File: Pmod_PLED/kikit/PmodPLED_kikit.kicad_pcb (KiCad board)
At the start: 2 copper layers, 88.5 x 101.3 mm, 212 parts, among them IC1 TBD62064APG, IC2 LM2940T-5.0, J1 Barrel_Jack_Switch, J3 Conn_01x03_Pin

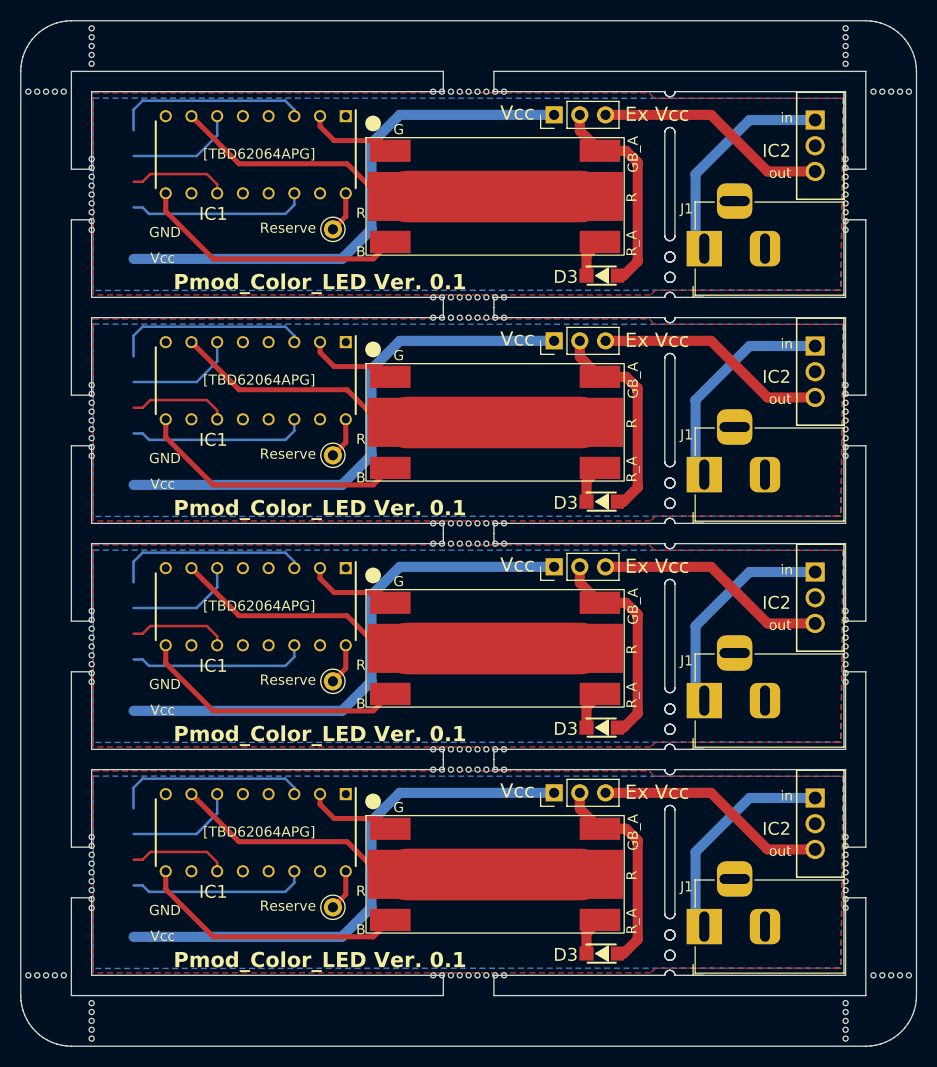
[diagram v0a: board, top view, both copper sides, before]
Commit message: 601
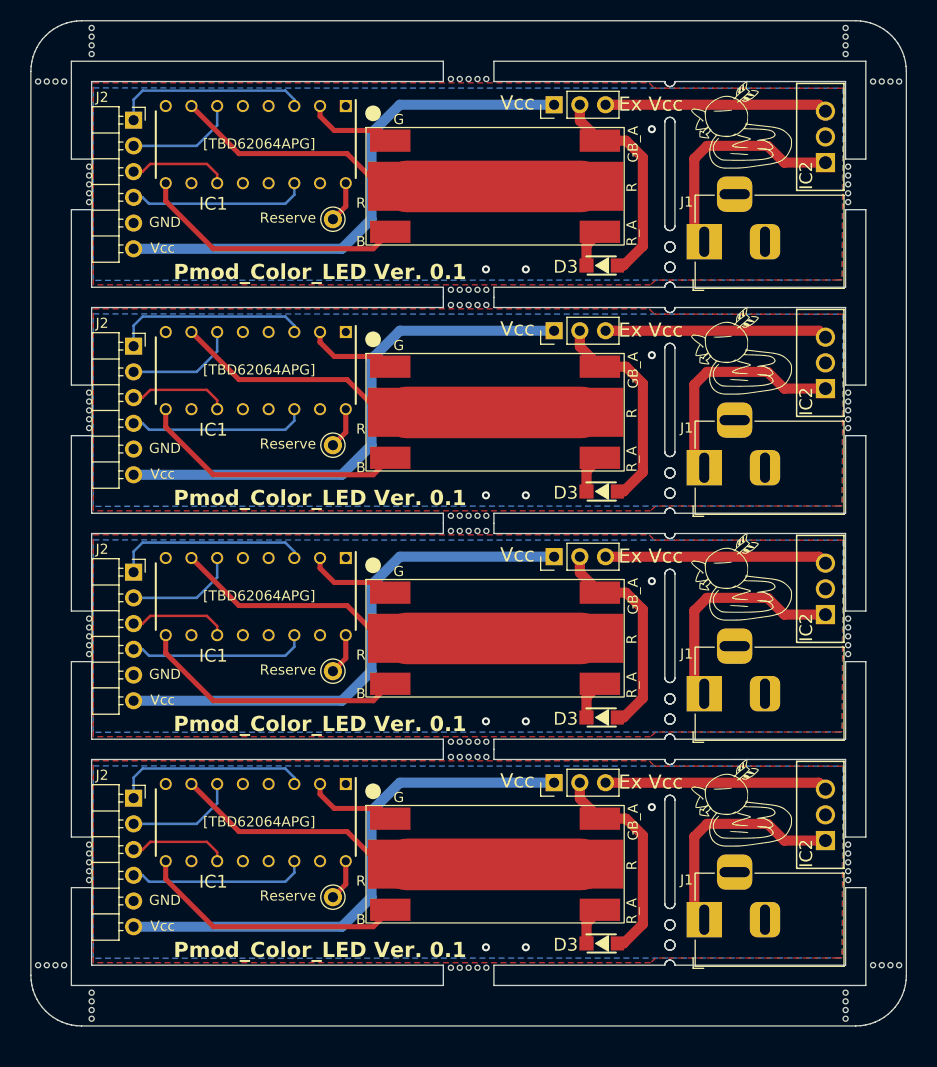
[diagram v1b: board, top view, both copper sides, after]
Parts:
- removed the D1 at (151.2, 104.3)
- removed the D1 at (151.2, 37.3)
- removed the D1 at (151.2, 59.7)
- removed the D1 at (151.2, 82.0)
- removed the D3 at (161.6, 45.2)
- removed the D3 at (161.6, 112.1)
- removed the D3 at (161.6, 89.8)
- removed the D3 at (161.6, 67.5)
- removed the IC1 at (127.5, 33.2)
- removed the IC1 at (127.5, 77.9)
- removed the IC1 at (127.5, 100.2)
- removed the IC1 at (127.5, 55.5)
- removed the IC2 at (183.7, 57.2)
- removed the IC2 at (183.7, 34.9)
- removed the IC2 at (183.7, 79.5)
- removed the IC2 at (183.7, 101.8)
- removed the J1 at (171.8, 42.5)
- removed the J1 at (171.8, 87.1)
- removed the J1 at (171.8, 109.5)
- removed the J1 at (171.8, 64.8)
- removed the J3 at (156.9, 96.2)
- removed the J3 at (156.9, 29.3)
- removed the J3 at (156.9, 73.9)
- removed the J3 at (156.9, 51.6)
- removed the REF** at (147.6, 47.3)
- removed the REF** at (111.3, 105.9)
- removed the REF** at (148.5, 47.3)
- removed the REF** at (111.3, 36.3)
- removed the REF** at (185.7, 58.6)
- removed the REF** at (147.6, 71.6)
- removed the REF** at (111.3, 63.0)
- removed the REF** at (150.2, 94.0)
- removed the REF** at (149.4, 92.0)
- removed the REF** at (185.7, 104.1)
- removed the REF** at (147.6, 49.3)
- removed the REF** at (145.0, 49.3)
- removed the REF** at (151.1, 71.6)
- removed the REF** at (145.0, 114.3)
- removed the REF** at (152.0, 71.6)
- removed the REF** at (111.3, 23.4)
- removed the REF** at (148.5, 94.0)
- removed the REF** at (192.0, 114.3)
- removed the REF** at (147.6, 94.0)
- removed the REF** at (185.7, 80.9)
- removed the REF** at (111.3, 33.7)
- removed the REF** at (148.5, 49.3)
- removed the REF** at (185.7, 85.3)
- removed the REF** at (145.9, 47.3)
- removed the REF** at (185.7, 84.4)
- removed the REF** at (111.3, 80.9)
- removed the REF** at (107.6, 114.3)
- removed the REF** at (190.2, 27.0)
- removed the REF** at (185.7, 81.8)
- removed the REF** at (111.3, 82.7)
- removed the REF** at (150.2, 27.0)
- removed the REF** at (152.0, 114.3)
- removed the REF** at (185.7, 118.8)
- removed the REF** at (145.0, 27.0)
- removed the REF** at (111.3, 118.8)
- removed the REF** at (150.2, 114.3)
- removed the REF** at (185.7, 119.6)
- removed the REF** at (145.0, 69.6)
- removed the REF** at (111.3, 79.2)
- removed the REF** at (146.8, 47.3)
- removed the REF** at (185.7, 20.8)
- removed the REF** at (185.7, 117.9)
- removed the REF** at (185.7, 38.9)
- removed the REF** at (189.4, 114.3)
- removed the REF** at (185.7, 103.2)
- removed the REF** at (185.7, 100.6)
- removed the REF** at (111.3, 57.7)
- removed the REF** at (185.7, 61.2)
- removed the REF** at (111.3, 62.1)
- removed the REF** at (152.0, 69.6)
- removed the REF** at (145.9, 94.0)
- removed the REF** at (146.8, 94.0)
- removed the REF** at (150.2, 71.6)
- removed the REF** at (152.0, 94.0)
- removed the REF** at (111.3, 21.6)
- removed the REF** at (145.9, 49.3)
- removed the REF** at (111.3, 102.4)
- removed the REF** at (111.3, 81.8)
- removed the REF** at (152.0, 27.0)
- removed the REF** at (111.3, 84.4)
- removed the REF** at (111.3, 101.5)
- removed the REF** at (147.6, 114.3)
- removed the REF** at (145.0, 94.0)
- removed the REF** at (111.3, 38.0)
- removed the REF** at (111.3, 24.2)
- removed the REF** at (191.1, 114.3)
- removed the REF** at (147.6, 92.0)
- removed the REF** at (188.5, 27.0)
- removed the REF** at (146.8, 49.3)
- removed the REF** at (111.3, 56.0)
- removed the REF** at (145.0, 47.3)
- removed the REF** at (111.3, 38.9)
- removed the REF** at (150.2, 69.6)
- removed the REF** at (185.7, 38.0)
- removed the REF** at (146.8, 92.0)
- removed the REF** at (185.7, 57.7)
- removed the REF** at (148.5, 92.0)
- removed the REF** at (185.7, 23.4)
- removed the REF** at (185.7, 107.6)
- removed the REF** at (149.4, 49.3)
- removed the REF** at (185.7, 35.4)
- removed the REF** at (185.7, 83.5)
- removed the REF** at (152.0, 92.0)
- removed the REF** at (111.3, 34.5)
- removed the REF** at (111.3, 39.8)
- removed the REF** at (185.7, 33.7)
- removed the REF** at (148.5, 69.6)
- removed the REF** at (151.1, 94.0)
- removed the REF** at (149.4, 69.6)
- removed the REF** at (147.6, 69.6)
- removed the REF** at (149.4, 71.6)
- removed the REF** at (185.7, 101.5)
- removed the REF** at (185.7, 21.6)
- removed the REF** at (146.8, 71.6)
- removed the REF** at (106.8, 27.0)
- removed the REF** at (151.1, 49.3)
- removed the REF** at (151.1, 47.3)
- removed the REF** at (185.7, 80.0)
- removed the REF** at (111.3, 107.6)
- removed the REF** at (146.8, 27.0)
- removed the REF** at (185.7, 39.8)
- removed the REF** at (149.4, 27.0)
- removed the REF** at (150.2, 92.0)
- removed the REF** at (111.3, 78.3)
- removed the REF** at (111.3, 60.4)
- removed the REF** at (111.3, 117.9)
- removed the REF** at (105.0, 27.0)
- removed the REF** at (111.3, 20.8)
- removed the REF** at (145.9, 114.3)
- removed the REF** at (185.7, 105.0)
- removed the REF** at (185.7, 40.7)
- removed the REF** at (145.9, 71.6)
- removed the REF** at (145.9, 69.6)
- removed the REF** at (148.5, 27.0)
- removed the REF** at (185.7, 106.7)
- removed the REF** at (145.0, 92.0)
- removed the REF** at (111.3, 106.7)
- removed the REF** at (190.2, 114.3)
- removed the REF** at (192.0, 27.0)
- removed the REF** at (189.4, 27.0)
- removed the REF** at (188.5, 114.3)
- removed the REF** at (185.7, 117.0)
- removed the REF** at (191.1, 27.0)
- removed the REF** at (185.7, 60.4)
- removed the REF** at (185.7, 22.5)
- removed the REF** at (149.4, 47.3)
- removed the REF** at (111.3, 37.2)
- removed the REF** at (185.7, 79.2)
- removed the REF** at (148.5, 114.3)
- removed the REF** at (185.7, 56.9)
- removed the REF** at (150.2, 49.3)
- removed the REF** at (185.7, 102.4)
- removed the REF** at (185.7, 62.1)
- removed the REF** at (185.7, 34.5)
- removed the REF** at (105.9, 27.0)
- removed the REF** at (150.2, 47.3)
- removed the REF** at (111.3, 104.1)
- removed the REF** at (149.4, 94.0)
- removed the REF** at (105.0, 114.3)
- removed the REF** at (147.6, 27.0)
- removed the REF** at (185.7, 24.2)
- removed the REF** at (185.7, 56.0)
- removed the REF** at (111.3, 35.4)
- removed the REF** at (108.5, 114.3)
- removed the REF** at (106.8, 114.3)
- removed the REF** at (105.9, 114.3)
- removed the REF** at (152.0, 49.3)
- removed the REF** at (111.3, 85.3)
- removed the REF** at (185.7, 36.3)
- removed the REF** at (185.7, 63.0)
- removed the REF** at (111.3, 59.5)
- removed the REF** at (107.6, 27.0)
- removed the REF** at (111.3, 40.7)
- removed the REF** at (185.7, 82.7)
- removed the REF** at (185.7, 105.9)
- removed the REF** at (146.8, 69.6)
- removed the REF** at (152.0, 47.3)
- removed the REF** at (111.3, 83.5)
- removed the REF** at (111.3, 100.6)
- removed the REF** at (111.3, 103.2)
- removed the REF** at (148.5, 71.6)
- removed the REF** at (111.3, 56.9)
- removed the REF** at (151.1, 114.3)
- removed the REF** at (185.7, 120.5)
- removed the REF** at (108.5, 27.0)
- removed the REF** at (111.3, 119.6)
- removed the REF** at (185.7, 78.3)
- removed the REF** at (145.0, 71.6)
- removed the REF** at (145.9, 27.0)
- removed the REF** at (146.8, 114.3)
- removed the REF** at (185.7, 37.2)
- removed the REF** at (145.9, 92.0)
- removed the REF** at (111.3, 22.5)
- removed the REF** at (111.3, 117.0)
- removed the REF** at (111.3, 120.5)
- removed the REF** at (111.3, 105.0)
- removed the REF** at (151.1, 27.0)
- removed the REF** at (111.3, 58.6)
- removed the REF** at (149.4, 114.3)
- removed the REF** at (185.7, 59.5)
- removed the REF** at (151.1, 92.0)
- removed the REF** at (111.3, 80.0)
- removed the REF** at (111.3, 61.2)
- removed the REF** at (151.1, 69.6)
- removed the Reserve at (135.1, 107.6)
- removed the Reserve at (135.1, 62.9)
- removed the Reserve at (135.1, 85.2)
- removed the Reserve at (135.1, 40.6)
- added D1: [EP204K-150G1R1B1-CA], MyLibrary:EP204-150G1R1B1-CA, F.Cu at (151.2, 58.7)
- added D1: [EP204K-150G1R1B1-CA], MyLibrary:EP204-150G1R1B1-CA, F.Cu at (151.2, 103.3)
- added D1: [EP204K-150G1R1B1-CA], MyLibrary:EP204-150G1R1B1-CA, F.Cu at (151.2, 81.0)
- added D1: [EP204K-150G1R1B1-CA], MyLibrary:EP204-150G1R1B1-CA, F.Cu at (151.2, 36.3)
- added D3: SS2040FL, SamacSys_Parts:SODFL3618X108N, F.Cu at (161.6, 66.5)
- added D3: SS2040FL, SamacSys_Parts:SODFL3618X108N, F.Cu at (161.6, 111.1)
- added D3: SS2040FL, SamacSys_Parts:SODFL3618X108N, F.Cu at (161.6, 88.8)
- added D3: SS2040FL, SamacSys_Parts:SODFL3618X108N, F.Cu at (161.6, 44.2)
- added G***: LOGO, MyLibrary:logo_kamo_ss, F.Cu at (175.4, 97.3)
- added G***: LOGO, MyLibrary:logo_kamo_ss, F.Cu at (175.4, 30.3)
- added G***: LOGO, MyLibrary:logo_kamo_ss, F.Cu at (175.4, 75.0)
- added G***: LOGO, MyLibrary:logo_kamo_ss, F.Cu at (175.4, 52.6)
- added IC1: TBD62064APG, SamacSys_Parts:DIP762W60P254L1975H445Q16N, F.Cu at (127.5, 76.9)
- added IC1: TBD62064APG, SamacSys_Parts:DIP762W60P254L1975H445Q16N, F.Cu at (127.5, 99.2)
- added IC1: TBD62064APG, SamacSys_Parts:DIP762W60P254L1975H445Q16N, F.Cu at (127.5, 54.5)
- added IC1: TBD62064APG, SamacSys_Parts:DIP762W60P254L1975H445Q16N, F.Cu at (127.5, 32.2)
- added IC2: LM2940T-5.0, SamacSys_Parts:TO254P470X1016X2222-3P, F.Cu at (182.7, 73.6)
- added IC2: LM2940T-5.0, SamacSys_Parts:TO254P470X1016X2222-3P, F.Cu at (182.7, 28.9)
- added IC2: LM2940T-5.0, SamacSys_Parts:TO254P470X1016X2222-3P, F.Cu at (182.7, 51.2)
- added IC2: LM2940T-5.0, SamacSys_Parts:TO254P470X1016X2222-3P, F.Cu at (182.7, 95.9)
- added J1: Barrel_Jack_Switch, Connector_BarrelJack:BarrelJack_Horizontal, F.Cu at (171.8, 86.5)
- added J1: Barrel_Jack_Switch, Connector_BarrelJack:BarrelJack_Horizontal, F.Cu at (171.8, 108.8)
- added J1: Barrel_Jack_Switch, Connector_BarrelJack:BarrelJack_Horizontal, F.Cu at (171.8, 64.1)
- added J1: Barrel_Jack_Switch, Connector_BarrelJack:BarrelJack_Horizontal, F.Cu at (171.8, 41.8)
- added J2: Conn_01x06_Pin, Library:Pmod6, F.Cu at (111.4, 28.5)
- added J2: Conn_01x06_Pin, Library:Pmod6, F.Cu at (111.4, 73.2)
- added J2: Conn_01x06_Pin, Library:Pmod6, F.Cu at (111.4, 50.9)
- added J2: Conn_01x06_Pin, Library:Pmod6, F.Cu at (111.4, 95.5)
- added J3: Conn_01x03_Pin, Connector_PinHeader_2.54mm:PinHeader_1x03_P2.54mm_Vertical, F.Cu at (156.9, 72.9)
- added J3: Conn_01x03_Pin, Connector_PinHeader_2.54mm:PinHeader_1x03_P2.54mm_Vertical, F.Cu at (156.9, 50.6)
- added J3: Conn_01x03_Pin, Connector_PinHeader_2.54mm:PinHeader_1x03_P2.54mm_Vertical, F.Cu at (156.9, 28.3)
- added J3: Conn_01x03_Pin, Connector_PinHeader_2.54mm:PinHeader_1x03_P2.54mm_Vertical, F.Cu at (156.9, 95.2)
- added REF**: NPTH, NPTH, F.Cu at (111.0, 103.1)
- added REF**: NPTH, NPTH, F.Cu at (149.4, 48.1)
- added REF**: NPTH, NPTH, F.Cu at (186.0, 57.6)
- added REF**: NPTH, NPTH, F.Cu at (150.2, 70.4)
- added REF**: NPTH, NPTH, F.Cu at (190.2, 113.3)
- added REF**: NPTH, NPTH, F.Cu at (111.0, 37.9)
- added REF**: NPTH, NPTH, F.Cu at (191.0, 113.3)
- added REF**: NPTH, NPTH, F.Cu at (186.0, 80.8)
- added REF**: NPTH, NPTH, F.Cu at (147.6, 48.1)
- added REF**: NPTH, NPTH, F.Cu at (111.3, 116.8)
- added REF**: NPTH, NPTH, F.Cu at (188.4, 113.3)
- added REF**: NPTH, NPTH, F.Cu at (146.8, 113.5)
- added REF**: NPTH, NPTH, F.Cu at (111.0, 34.4)
- added REF**: NPTH, NPTH, F.Cu at (186.0, 82.5)
- added REF**: NPTH, NPTH, F.Cu at (147.6, 91.2)
- added REF**: NPTH, NPTH, F.Cu at (106.0, 26.0)
- added REF**: NPTH, NPTH, F.Cu at (150.2, 113.5)
- added REF**: NPTH, NPTH, F.Cu at (146.8, 68.9)
- added REF**: NPTH, NPTH, F.Cu at (186.0, 34.4)
- added REF**: NPTH, NPTH, F.Cu at (150.2, 25.8)
- added REF**: NPTH, NPTH, F.Cu at (148.5, 113.5)
- added REF**: NPTH, NPTH, F.Cu at (186.0, 104.0)
- added REF**: NPTH, NPTH, F.Cu at (185.7, 116.8)
- added REF**: NPTH, NPTH, F.Cu at (149.4, 25.8)
- added REF**: NPTH, NPTH, F.Cu at (106.0, 113.3)
- added REF**: NPTH, NPTH, F.Cu at (186.0, 36.2)
- added REF**: NPTH, NPTH, F.Cu at (111.0, 81.7)
- added REF**: NPTH, NPTH, F.Cu at (149.4, 70.4)
- added REF**: NPTH, NPTH, F.Cu at (111.0, 59.4)
- added REF**: NPTH, NPTH, F.Cu at (111.0, 35.3)
- added REF**: NPTH, NPTH, F.Cu at (189.3, 26.0)
- added REF**: NPTH, NPTH, F.Cu at (111.0, 60.2)
- added REF**: NPTH, NPTH, F.Cu at (108.6, 26.0)
- added REF**: NPTH, NPTH, F.Cu at (111.0, 37.0)
- added REF**: NPTH, NPTH, F.Cu at (186.0, 101.4)
- added REF**: NPTH, NPTH, F.Cu at (186.0, 102.2)
- added REF**: NPTH, NPTH, F.Cu at (186.0, 79.9)
- added REF**: NPTH, NPTH, F.Cu at (150.2, 68.9)
- added REF**: NPTH, NPTH, F.Cu at (111.0, 79.9)
- added REF**: NPTH, NPTH, F.Cu at (149.4, 92.7)
- added REF**: NPTH, NPTH, F.Cu at (191.0, 26.0)
- added REF**: NPTH, NPTH, F.Cu at (150.2, 91.2)
- added REF**: NPTH, NPTH, F.Cu at (188.4, 26.0)
- added REF**: NPTH, NPTH, F.Cu at (190.2, 26.0)
- added REF**: NPTH, NPTH, F.Cu at (150.2, 92.7)
- added REF**: NPTH, NPTH, F.Cu at (111.0, 104.9)
- added REF**: NPTH, NPTH, F.Cu at (111.3, 117.7)
- added REF**: NPTH, NPTH, F.Cu at (146.8, 46.6)
- added REF**: NPTH, NPTH, F.Cu at (111.0, 82.5)
- added REF**: NPTH, NPTH, F.Cu at (186.0, 79.0)
- added REF**: NPTH, NPTH, F.Cu at (146.8, 48.1)
- added REF**: NPTH, NPTH, F.Cu at (185.7, 117.7)
- added REF**: NPTH, NPTH, F.Cu at (148.5, 68.9)
- added REF**: NPTH, NPTH, F.Cu at (148.5, 25.8)
- added REF**: NPTH, NPTH, F.Cu at (146.8, 25.8)
- added REF**: NPTH, NPTH, F.Cu at (106.8, 26.0)
- added REF**: NPTH, NPTH, F.Cu at (149.4, 91.2)
- added REF**: NPTH, NPTH, F.Cu at (149.4, 46.6)
- added REF**: NPTH, NPTH, F.Cu at (111.3, 22.4)
- added REF**: NPTH, NPTH, F.Cu at (111.0, 36.2)
- added REF**: NPTH, NPTH, F.Cu at (146.8, 91.2)
- added REF**: NPTH, NPTH, F.Cu at (186.0, 35.3)
- added REF**: NPTH, NPTH, F.Cu at (111.3, 23.3)
- added REF**: NPTH, NPTH, F.Cu at (185.7, 23.3)
- added REF**: NPTH, NPTH, F.Cu at (149.4, 113.5)
- added REF**: NPTH, NPTH, F.Cu at (148.5, 46.6)
- added REF**: NPTH, NPTH, F.Cu at (150.2, 46.6)
- added REF**: NPTH, NPTH, F.Cu at (111.0, 57.6)
- added REF**: NPTH, NPTH, F.Cu at (108.6, 113.3)
- added REF**: NPTH, NPTH, F.Cu at (150.2, 48.1)
- added REF**: NPTH, NPTH, F.Cu at (111.0, 102.2)
- added REF**: NPTH, NPTH, F.Cu at (111.3, 21.6)
- added REF**: NPTH, NPTH, F.Cu at (148.5, 91.2)
- added REF**: NPTH, NPTH, F.Cu at (148.5, 92.7)
- added REF**: NPTH, NPTH, F.Cu at (111.0, 80.8)
- added REF**: NPTH, NPTH, F.Cu at (111.0, 104.0)
- added REF**: NPTH, NPTH, F.Cu at (186.0, 59.4)
- added REF**: NPTH, NPTH, F.Cu at (148.5, 70.4)
- added REF**: NPTH, NPTH, F.Cu at (111.3, 116.0)
- added REF**: NPTH, NPTH, F.Cu at (186.0, 58.5)
- added REF**: NPTH, NPTH, F.Cu at (185.7, 20.7)
- added REF**: NPTH, NPTH, F.Cu at (186.0, 37.9)
- added REF**: NPTH, NPTH, F.Cu at (147.6, 46.6)
- added REF**: NPTH, NPTH, F.Cu at (186.0, 60.2)
- added REF**: NPTH, NPTH, F.Cu at (186.0, 103.1)
- added REF**: NPTH, NPTH, F.Cu at (111.3, 118.6)
- added REF**: NPTH, NPTH, F.Cu at (186.0, 104.9)
- added REF**: NPTH, NPTH, F.Cu at (186.0, 37.0)
- added REF**: NPTH, NPTH, F.Cu at (185.7, 22.4)
- added REF**: NPTH, NPTH, F.Cu at (146.8, 70.4)
- added REF**: NPTH, NPTH, F.Cu at (186.0, 81.7)
- added REF**: NPTH, NPTH, F.Cu at (147.6, 113.5)
- added REF**: NPTH, NPTH, F.Cu at (185.7, 21.6)
- added REF**: NPTH, NPTH, F.Cu at (189.3, 113.3)
- added REF**: NPTH, NPTH, F.Cu at (147.6, 25.8)
- added REF**: NPTH, NPTH, F.Cu at (147.6, 70.4)
- added REF**: NPTH, NPTH, F.Cu at (185.7, 118.6)
- added REF**: NPTH, NPTH, F.Cu at (146.8, 92.7)
- added REF**: NPTH, NPTH, F.Cu at (111.3, 20.7)
- added REF**: NPTH, NPTH, F.Cu at (147.6, 68.9)
- added REF**: NPTH, NPTH, F.Cu at (147.6, 92.7)
- added REF**: NPTH, NPTH, F.Cu at (107.7, 26.0)
- added REF**: NPTH, NPTH, F.Cu at (111.0, 56.7)
- added REF**: NPTH, NPTH, F.Cu at (111.0, 58.5)
- added REF**: NPTH, NPTH, F.Cu at (149.4, 68.9)
- added REF**: NPTH, NPTH, F.Cu at (186.0, 56.7)
- added REF**: NPTH, NPTH, F.Cu at (106.8, 113.3)
- added REF**: NPTH, NPTH, F.Cu at (107.7, 113.3)
- added REF**: NPTH, NPTH, F.Cu at (111.0, 101.4)
- added REF**: NPTH, NPTH, F.Cu at (111.0, 79.0)
- added REF**: NPTH, NPTH, F.Cu at (185.7, 116.0)
- added REF**: NPTH, NPTH, F.Cu at (148.5, 48.1)
- added Reserve: TestPoint, TestPoint:TestPoint_Pad_D2.0mm, F.Cu at (135.1, 106.6)
- added Reserve: TestPoint, TestPoint:TestPoint_Pad_D2.0mm, F.Cu at (135.1, 84.2)
- added Reserve: TestPoint, TestPoint:TestPoint_Pad_D2.0mm, F.Cu at (135.1, 61.9)
- added Reserve: TestPoint, TestPoint:TestPoint_Pad_D2.0mm, F.Cu at (135.1, 39.6)
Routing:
- net Board_3-/ExVcc: track 23.0 -> 22.0 mm
- net Board_1-/ExVcc: track 23.0 -> 22.0 mm
- net Board_0-/ExVcc: track 23.0 -> 22.0 mm
- net Board_2-/ExVcc: track 23.0 -> 22.0 mm
- net Board_3-Net-(IC2-IN): track 21.7 -> 22.4 mm
- net Board_1-Net-(IC2-IN): track 21.7 -> 22.4 mm
- net Board_0-Net-(IC2-IN): track 21.7 -> 22.4 mm
- net Board_2-Net-(IC2-IN): track 21.7 -> 22.4 mm
- net Board_3-GND: vias 0 -> 3
- net Board_2-GND: vias 0 -> 3
- net Board_1-GND: vias 0 -> 3
- net Board_0-GND: vias 0 -> 3
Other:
- board size 88.5 x 101.3 mm -> 86.5 x 99.3 mm
